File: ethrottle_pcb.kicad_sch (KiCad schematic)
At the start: 49 parts

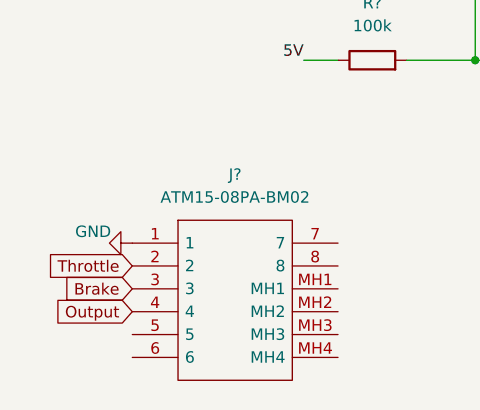
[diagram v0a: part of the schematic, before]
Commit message: update connections
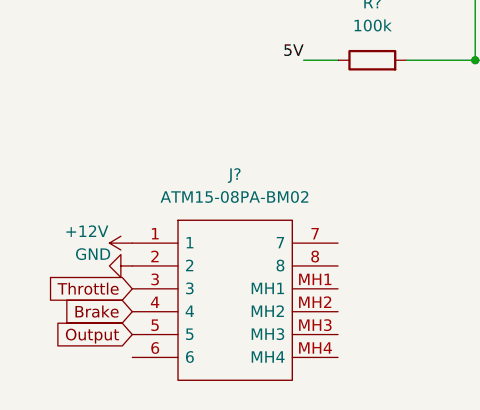
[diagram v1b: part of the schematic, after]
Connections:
- net +12V: now also J?.1
- net Brake: now also J?.4; no longer J?.2
- net GND: now also J?.2; no longer J?.1
- net Output: now also J?.5; no longer J?.4
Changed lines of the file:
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@@
     (effects (font (size 1.27 1.27)) (justify left bottom))
   )
-  (global_label "Throttle" (shape input) (at 31.75 132.08 180) (fields_autoplaced)
+  (global_label "Throttle" (shape input) (at 31.75 134.62 180) (fields_autoplaced)
     (effects (font (size 1.27 1.27)) (justify right))
-    (property "Intersheet References" "${INTERSHEET_REFS}" (id 0) (at 22.0798 132.1594 0)
+    (property "Intersheet References" "${INTERSHEET_REFS}" (id 0) (at 22.0798 134.6994 0)
       (effects (font (size 1.27 1.27)) (justify right) hide)
     )
@@
     )
   )
-  (global_label "Output" (shape input) (at 31.75 137.16 180) (fields_autoplaced)
+  (global_label "Output" (shape input) (at 31.75 139.7 180) (fields_autoplaced)
     (effects (font (size 1.27 1.27)) (justify right))
-    (property "Intersheet References" "${INTERSHEET_REFS}" (id 0) (at 23.1079 137.0806 0)
+    (property "Intersheet References" "${INTERSHEET_REFS}" (id 0) (at 23.1079 139.6206 0)
       (effects (font (size 1.27 1.27)) (justify right) hide)
     )
@@
     )
   )
-  (global_label "Brake" (shape input) (at 31.75 134.62 180) (fields_autoplaced)
+  (global_label "Brake" (shape input) (at 31.75 137.16 180) (fields_autoplaced)
     (effects (font (size 1.27 1.27)) (justify right))
-    (property "Intersheet References" "${INTERSHEET_REFS}" (id 0) (at 24.015 134.5406 0)
+    (property "Intersheet References" "${INTERSHEET_REFS}" (id 0) (at 24.015 137.0806 0)
       (effects (font (size 1.27 1.27)) (justify right) hide)
     )
@@
     (pin "2")
   )
+  (symbol (lib_id "power:+12V") (at 31.75 129.54 90) (unit 1)
+    (in_bom yes) (on_board yes)
+    (property "Reference" "#PWR?" (id 0) (at 35.56 129.54 0)
+      (effects (font (size 1.27 1.27)) hide)
+    )
+    (property "Value" "+12V" (id 1) (at 26.67 128.27 90))
+    (property "Footprint" "" (id 2) (at 31.75 129.54 0)
+      (effects (font (size 1.27 1.27)) hide)
+    )
+    (property "Datasheet" "" (id 3) (at 31.75 129.54 0)
+      (effects (font (size 1.27 1.27)) hide)
+    )
+    (pin "1")
+  )
   (symbol (lib_id "Device:R") (at 167.64 45.72 0) (unit 1)
     (in_bom yes) (on_board yes) (fields_autoplaced)
@@
     (pin "4")
   )
-  (symbol (lib_id "power:GND") (at 31.75 129.54 270) (unit 1)
-    (in_bom yes) (on_board yes)
-    (property "Reference" "#PWR?" (id 0) (at 25.4 129.54 0)
-      (effects (font (size 1.27 1.27)) hide)
-    )
-    (property "Value" "GND" (id 1) (at 25.4 128.27 90)
-      (effects (font (size 1.27 1.27)) (justify left))
-    )
-    (property "Footprint" "" (id 2) (at 31.75 129.54 0)
-      (effects (font (size 1.27 1.27)) hide)
-    )
-    (property "Datasheet" "" (id 3) (at 31.75 129.54 0)
+  (symbol (lib_id "power:GND") (at 31.75 132.08 270) (unit 1)
+    (in_bom yes) (on_board yes)
+    (property "Reference" "#PWR?" (id 0) (at 25.4 132.08 0)
+      (effects (font (size 1.27 1.27)) hide)
+    )
+    (property "Value" "GND" (id 1) (at 25.4 130.81 90)
+      (effects (font (size 1.27 1.27)) (justify left))
+    )
+    (property "Footprint" "" (id 2) (at 31.75 132.08 0)
+      (effects (font (size 1.27 1.27)) hide)
+    )
+    (property "Datasheet" "" (id 3) (at 31.75 132.08 0)
       (effects (font (size 1.27 1.27)) hide)
     )
@@
       (reference "#PWR?") (unit 1) (value "GND") (footprint "")
     )
+    (path "/af4fe4c5-3121-44b8-959e-e5c992990974"
+      (reference "#PWR?") (unit 1) (value "+12V") (footprint "")
+    )
     (path "/c3affea8-6cb9-4035-a7f6-fd73cd47eeb6"

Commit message: update footprints
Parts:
- C?: footprint (none) -> Capacitor_SMD:C_0805_2012Metric
- R? (x22): footprint (none) -> Resistor_SMD:R_01005_0402Metric
